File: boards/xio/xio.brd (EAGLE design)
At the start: 170 x 170 mm, 286 parts, among them CN3 J00-0065NL, U2 LAN8742A-CZ, X2 USB-A, Y1 NX3225SA-12.000MHZ-STD-CSR-1, Y2 NX3225SA-12.000MHZ-STD-CSR-1, Y3 NX3225SA-25.000MHZ-STD-CSR-1

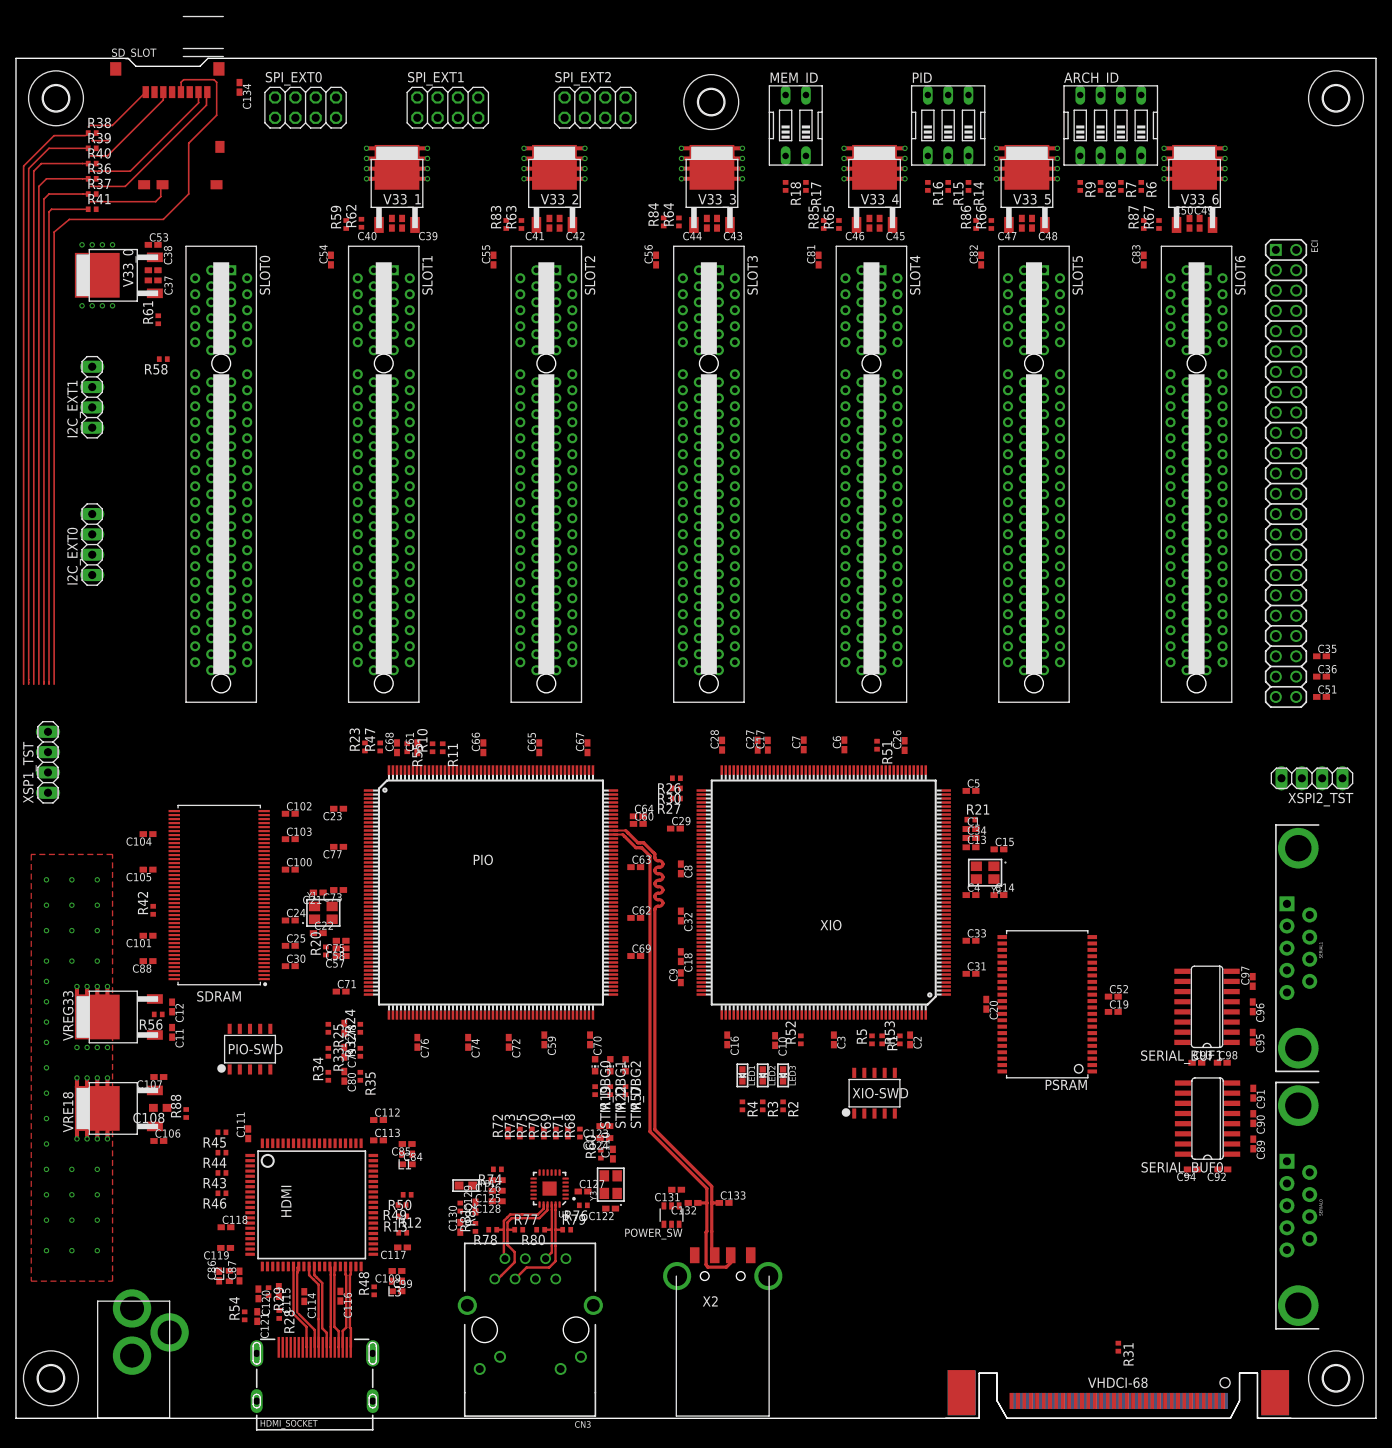
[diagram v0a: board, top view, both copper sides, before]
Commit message: Latest schematic/board after most things in the review completed
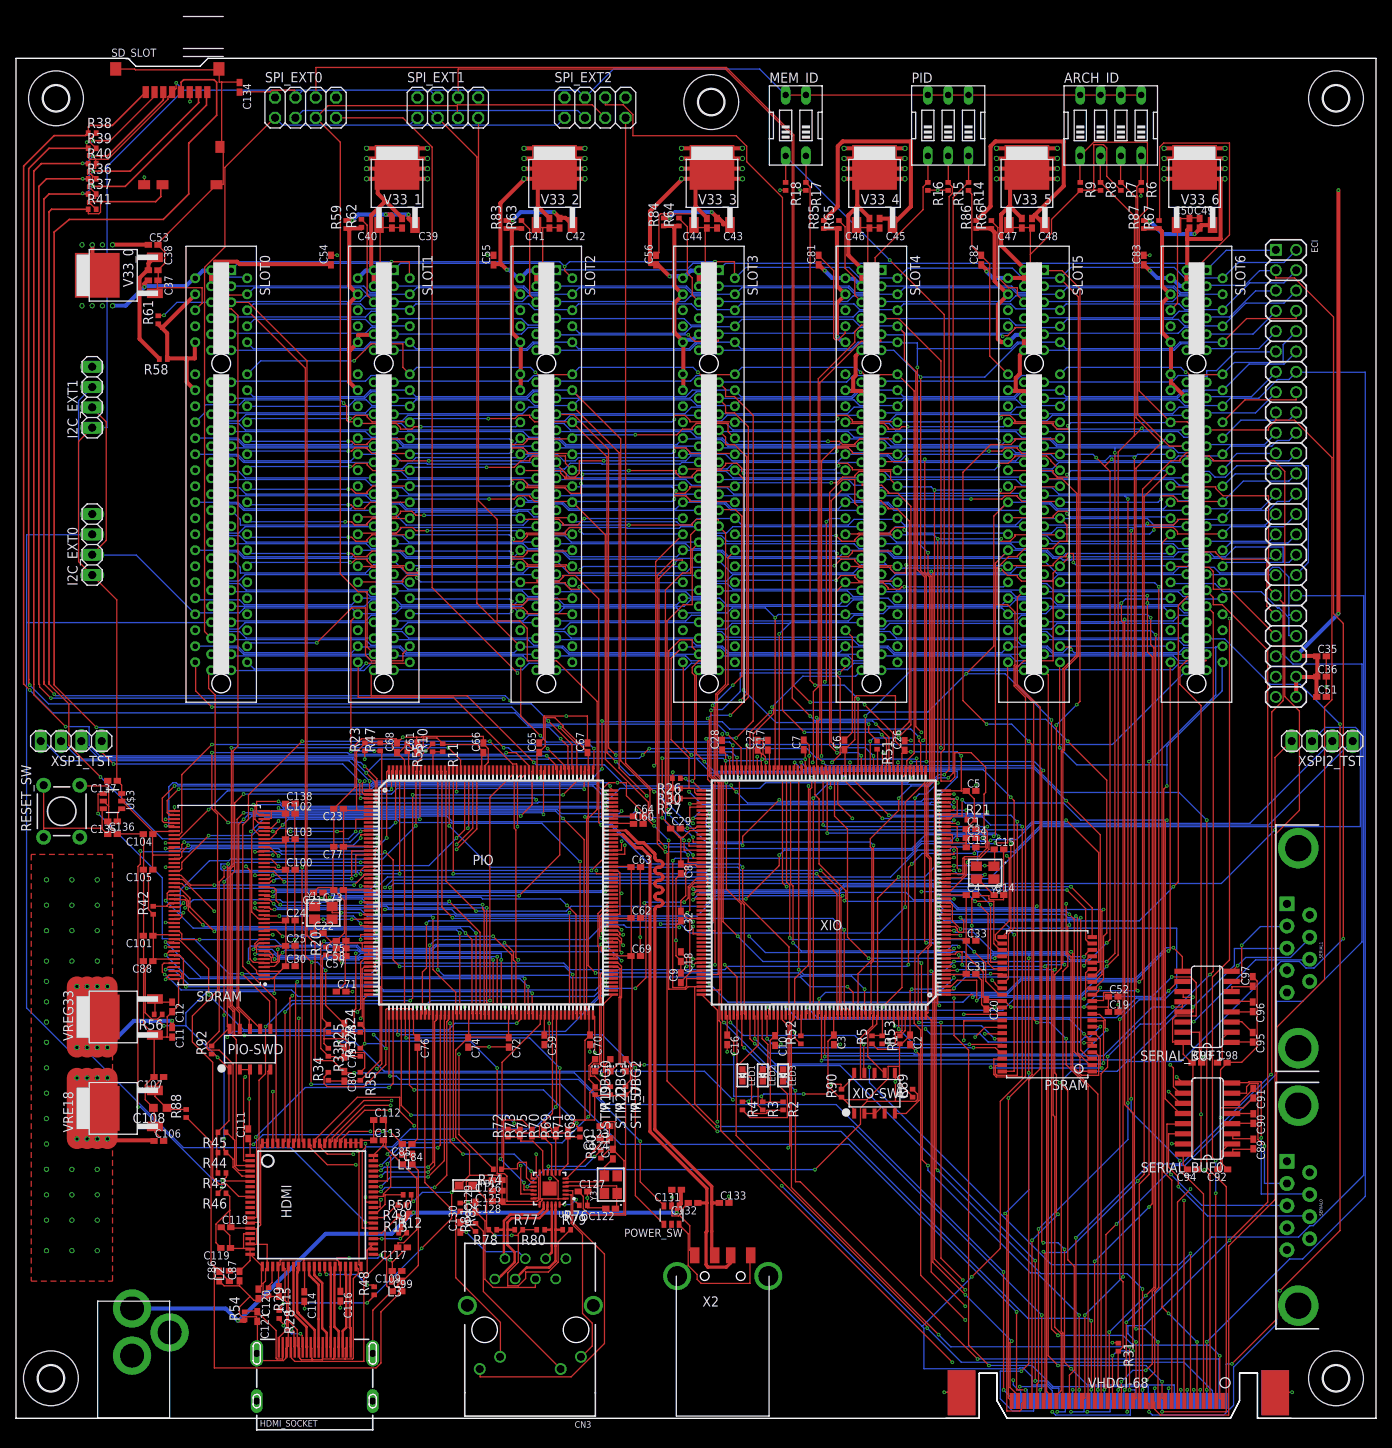
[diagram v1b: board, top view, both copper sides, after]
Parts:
- added C135: 120pF, rcl:C0402K
- added C136: 10nF, rcl:C0402K
- added C137: 0.1uF, rcl:C0402K
- added C138: 4.7uF, rcl:C0402K
- added R89, R90, R92: 10K, rcl:R0402
- added RESET_SW: (no value), SparkFun:TACTILE-PTH
- added U$3: TPS3808G33DBVR, sjg-power:SOT23-6
- moved XSPI2_TST 4.82 mm to (163.3, 84.6)
- moved XSP1_TST 3.93 mm to (6.90, 84.6), turned to 180 degrees
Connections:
- net N$128 renamed PIO_RX
- net N$129 renamed PIO_TX
- net N$130 renamed PIO_SWDCLK
- removed net N$131: PIO-SWD.P2, PIO.147
- new net !MR!: C136.1, RESET_SW.1, RESET_SW.2, U$3.3
- new net N$60: C135.1, U$3.4
- new net PIO_SWDIO: PIO-SWD.P2, PIO.147, R92.2
- net !RESET!: now also R89.2, U$3.1
- net +3V3: now also C137.1, C138.1, R89.1, R90.1, R92.1, U$3.5, U$3.6
- net GND: now also C135.2, C136.2, C137.2, C138.2, RESET_SW.3, RESET_SW.4, U$3.2
- net XIO_SWDIO: now also R90.2
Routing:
- net +3V3: track 0.00 -> 1151.8 mm, vias 0 -> 33
- net GND: track 0.00 -> 879.4 mm, vias 0 -> 83
- net +5V: track 127.4 -> 540.4 mm, vias 104 -> 116
- net VHDCI_AUDIO_SIO: track 0.00 -> 359.8 mm, vias 0 -> 5
- net VHDCI_A9: track 0.00 -> 356.9 mm, vias 0 -> 4
- net VHDCI_A2: track 0.00 -> 352.0 mm, vias 0 -> 6
- net VHDCI_A12: track 0.00 -> 345.3 mm, vias 0 -> 3
- net VHDCI_AUDIO_L: track 0.00 -> 342.1 mm, vias 0 -> 4
- net VHDCI_AUDIO_R: track 0.00 -> 340.3 mm, vias 0 -> 3
- net I2C_SDA: track 0.00 -> 336.8 mm, vias 0 -> 3
- net !VHDCI_MPD!: track 0.00 -> 331.1 mm, vias 0 -> 3
- net VHDCI_D2: track 0.00 -> 330.3 mm, vias 0 -> 5
- net VHDCI_A11: track 0.00 -> 320.6 mm, vias 0 -> 10
- net VHDCI_REF: track 0.00 -> 316.4 mm, vias 0 -> 4
- net VHDCI_A10: track 0.00 -> 311.8 mm, vias 0 -> 3
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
